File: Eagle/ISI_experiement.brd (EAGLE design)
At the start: 100 x 81.7 mm, 59 parts, among them IC1 74AC11374D, IC3 74AC11374D, IC4 74AC11374D, IC5 74266D, IC6 74266D, IC7 74HC04D

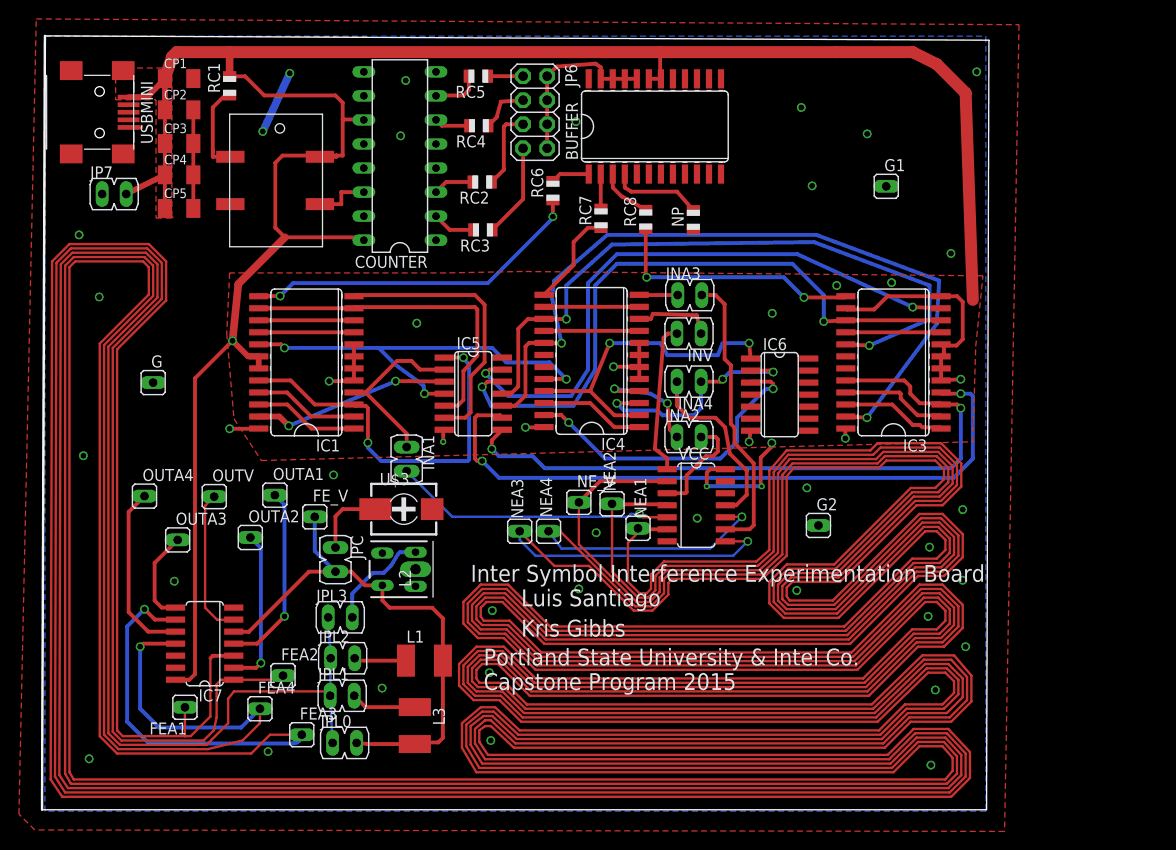
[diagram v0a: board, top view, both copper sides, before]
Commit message: test board included
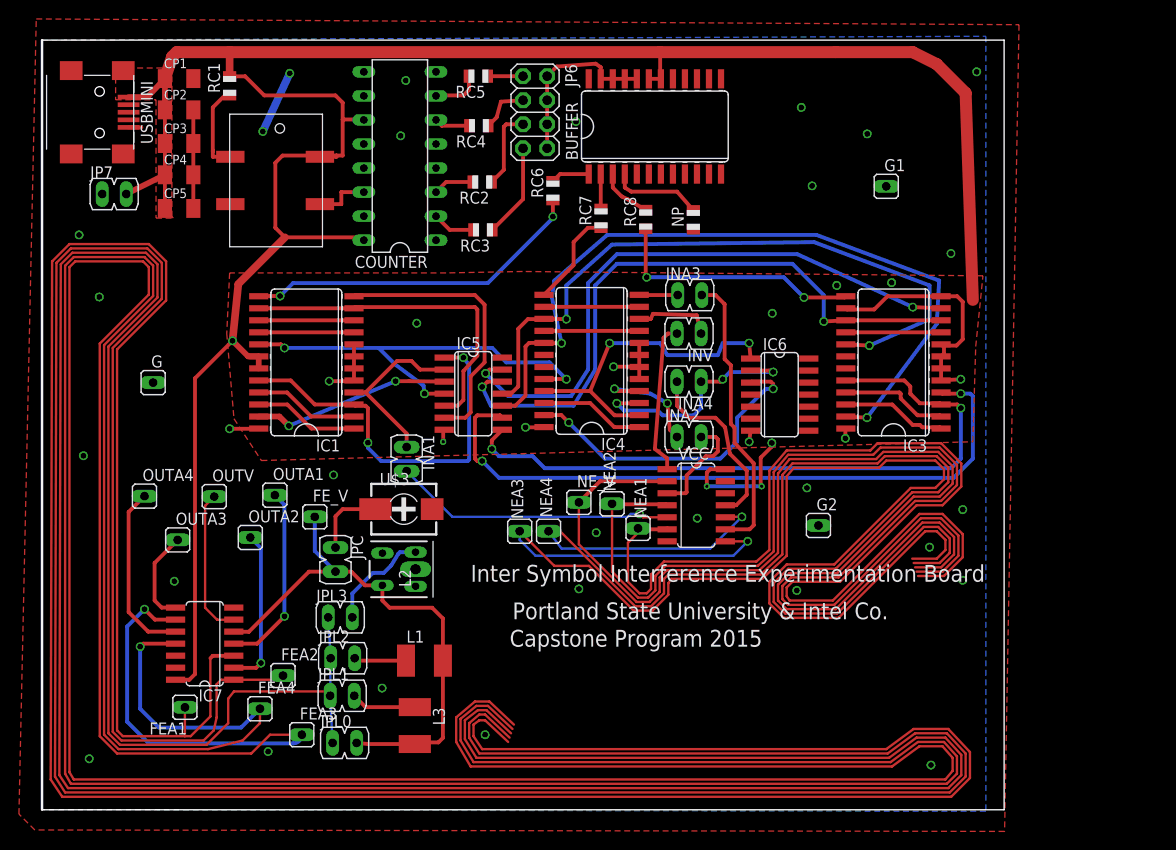
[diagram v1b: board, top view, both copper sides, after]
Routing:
- net 4: track 698.7 -> 421.4 mm
- net 2: track 702.2 -> 425.2 mm
- net V1: track 722.6 -> 446.0 mm
- net 1: track 735.6 -> 459.4 mm
- net 3: track 754.0 -> 478.2 mm
- net GND: vias 44 -> 39
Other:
- board size 100 x 81.7 mm -> 101.6 x 81.3 mm
- board text removed: "Kris Gibbs"
- board text removed: "Luis Santiago"
